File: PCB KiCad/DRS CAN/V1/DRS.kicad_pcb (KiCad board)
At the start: 2 copper layers, 70 x 46.5 mm, 39 parts, among them J1 Screw_Terminal_01x02, J2 Screw_Terminal_01x02, J3 Conn_02x03_Odd_Even, J4 Conn_01x03_Male, J5 Screw_Terminal_01x04, SW1 SW_Push, SW2 SW_Push, SW3 SW_Push, U1 AT90CAN32-16AU, U2 MCP2562-E-SN, U3 LM2596S-5, Y1 Crystal

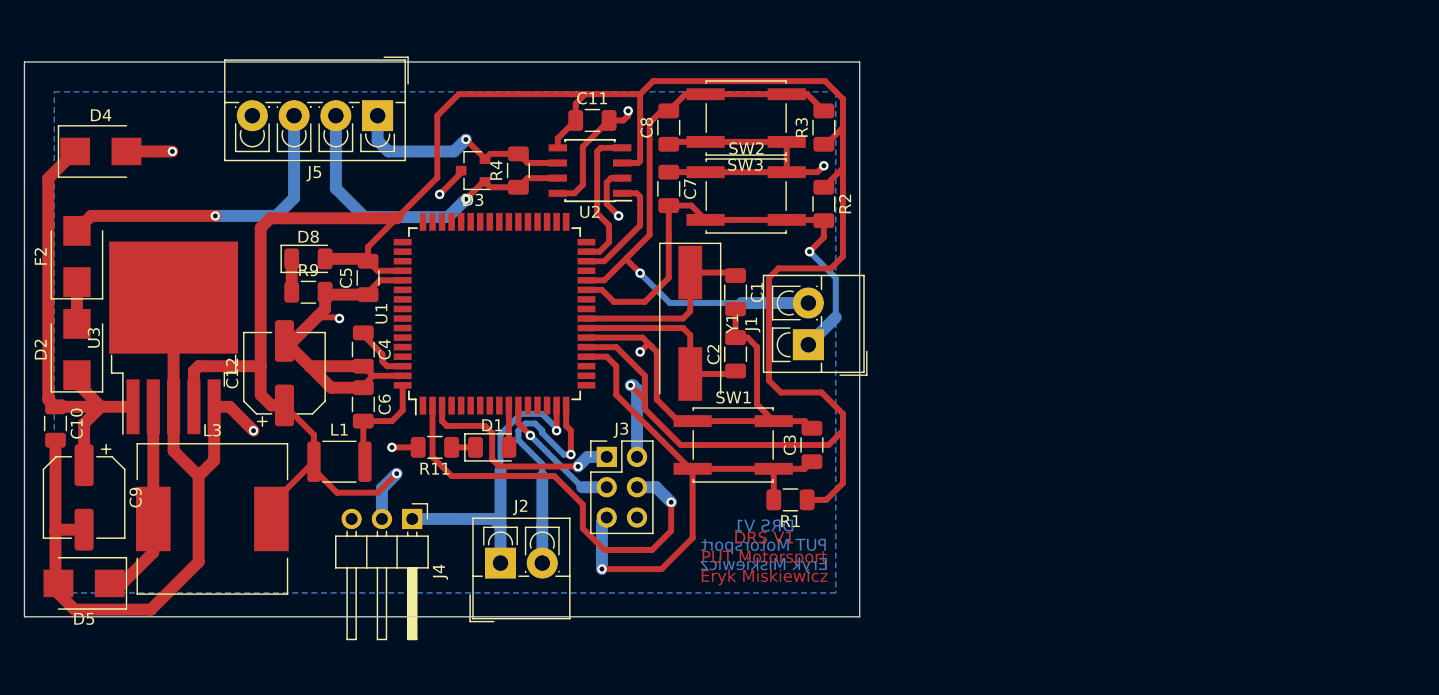
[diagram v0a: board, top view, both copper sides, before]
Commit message: WersjaV2 PCB
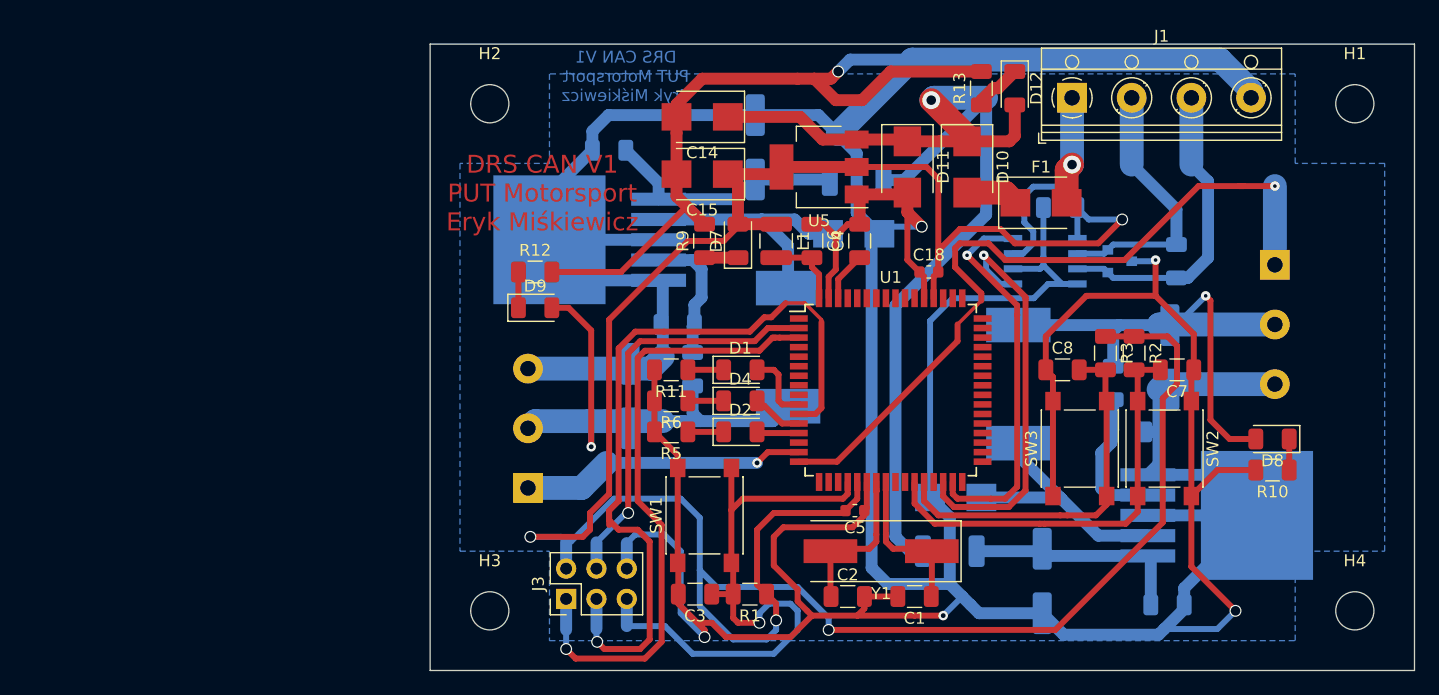
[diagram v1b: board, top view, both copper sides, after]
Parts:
- removed F2: Fuse, Diode_SMD:D_SMB
- removed J5: Screw_Terminal_01x04, TerminalBlock_4Ucon:TerminalBlock_4Ucon_1x04_P3.50mm_Vertical
- added C13: 100n, Capacitor_SMD:C_1206_3216Metric, B.Cu at (109.0, 59.9)
- added C14: CP, Diode_SMD:D_SMB, F.Cu at (116.8, 57.1)
- added C15: CP, Diode_SMD:D_SMB, F.Cu at (116.8, 61.9)
- added C16: 220u, Capacitor_SMD:CP_Elec_6.3x7.7, B.Cu at (156.0, 77.2)
- added C17: 220u, Capacitor_SMD:CP_Elec_6.3x7.7, B.Cu at (110.8, 80.5)
- added C18: 100n, Capacitor_SMD:C_0603_1608Metric, F.Cu at (135.8, 70.1)
- added D10: D_Schottky, Diode_SMD:D_SMB, F.Cu at (139.0, 61.3)
- added D11: D_Zener, Diode_SMD:D_SMB, F.Cu at (134.0, 61.3)
- added D12: LED, LED_SMD:LED_1206_3216Metric, F.Cu at (143.0, 54.7)
- added D6: D_Schottky, Diode_SMD:D_SMB, B.Cu at (129.5, 66.9)
- added D7: LED, LED_SMD:LED_1206_3216Metric, F.Cu at (119.8, 67.5)
- added D9: LED, LED_SMD:LED_1206_3216Metric, F.Cu at (102.8, 73.1)
- added F1: Fuse, Diode_SMD:D_SMB, F.Cu at (145.2, 64.3)
- added H1: MountingHole, MountingHole:MountingHole_3.2mm_M3, F.Cu at (171.5, 56.0)
- added H2: MountingHole, MountingHole:MountingHole_3.2mm_M3, F.Cu at (99.0, 56.0)
- added H3: MountingHole, MountingHole:MountingHole_3.2mm_M3, F.Cu at (99.0, 98.5)
- added H4: MountingHole, MountingHole:MountingHole_3.2mm_M3, F.Cu at (171.5, 98.5)
- added L2: 33u, Inductor_SMD:L_12x12mm_H8mm, B.Cu at (143.3, 79.5)
- added R10: 330, Resistor_SMD:R_1206_3216Metric, F.Cu at (164.6, 86.7)
- added R12: 330, Resistor_SMD:R_1206_3216Metric, F.Cu at (102.8, 70.1)
- added R13: 2k, Resistor_SMD:R_1206_3216Metric, F.Cu at (140.2, 54.7)
- added R14: 0R, Resistor_SMD:R_1206_3216Metric, B.Cu at (152.5, 83.5)
- added R15: 0R, Resistor_SMD:R_1206_3216Metric, B.Cu at (114.8, 74.5)
- added R16: 0R, Resistor_SMD:R_1206_3216Metric, B.Cu at (151.2, 79.4)
- added R17: 0R, Resistor_SMD:R_1206_3216Metric, B.Cu at (116.0, 78.2)
- added R5: 330, Resistor_SMD:R_1206_3216Metric, F.Cu at (114.2, 83.5)
- added R6: 330, Resistor_SMD:R_1206_3216Metric, F.Cu at (114.2, 80.9)
- added R7: 0R, Resistor_SMD:R_2010_5025Metric, B.Cu at (129.8, 62.4)
- added R8: 0R, Resistor_SMD:R_2010_5025Metric, B.Cu at (137.6, 93.5)
- added U4: AP1501-K5G-13, Package_TO_SOT_SMD:TO-263-5_TabPin3, B.Cu at (107.4, 67.4)
- added U5: LM1117-5.0, Package_TO_SOT_SMD:SOT-223-3_TabPin2, F.Cu at (126.6, 61.3)
- C10: value 100n -> 100u; footprint Capacitor_SMD:C_1206_3216Metric -> Capacitor_SMD:CP_Elec_6.3x7.7; moved to B.Cu
- C11, C9, D3, D5, L3, R4, U2: moved to B.Cu
- C12: value 470u/220u -> 100n; footprint Capacitor_SMD:CP_Elec_6.3x7.7 -> Capacitor_SMD:C_1206_3216Metric; moved to B.Cu
- C5: footprint Capacitor_SMD:C_1206_3216Metric -> Capacitor_SMD:C_0603_1608Metric
- D2: value D_Schottky -> LED; footprint Diode_SMD:D_SMB -> LED_SMD:LED_1206_3216Metric
- D4: value D_Zener -> LED; footprint Diode_SMD:D_SMB -> LED_SMD:LED_1206_3216Metric
- J1: value Screw_Terminal_01x02 -> Screw_Terminal_01x04; footprint TerminalBlock_4Ucon:TerminalBlock_4Ucon_1x02_P3.50mm_Vertical -> TerminalBlock_RND:TerminalBlock_RND_205-00014_1x04_P5.00mm_Horizontal
- J2: value Screw_Terminal_01x02 -> Screw_Terminal_01x03; footprint TerminalBlock_4Ucon:TerminalBlock_4Ucon_1x02_P3.50mm_Vertical -> TerminalBlock_RND:TerminalBlock_RND_205-00013_1x03_P5.00mm_Horizontal; moved to B.Cu
- J4: value Conn_01x03_Male -> Screw_Terminal_01x03; footprint Connector_PinHeader_2.54mm:PinHeader_1x03_P2.54mm_Horizontal -> TerminalBlock_RND:TerminalBlock_RND_205-00013_1x03_P5.00mm_Horizontal; moved to B.Cu
- L1: footprint Inductor_SMD:L_1812_4532Metric -> Inductor_SMD:L_1210_3225Metric
- R2, R3: value R -> 10k
- SW1, SW2, SW3: footprint Button_Switch_SMD:SW_SPST_EVQQ2 -> Button_Switch_SMD:SW_SPST_PTS645
- U3: value LM2596S-5 -> AP1501-K5G-13; moved to B.Cu
- moved U3 88.7 mm to (159.9, 90.5), turned to 0 degrees
- moved D8 82.2 mm to (164.6, 84.1), turned to 180 degrees
- moved C9 80.6 mm to (145.3, 96.0)
- moved C12 76.5 mm to (155.8, 98.0), turned to 0 degrees
- moved J4 75.4 mm to (164.8, 69.5)
- moved D5 73.4 mm to (138.1, 89.0)
- moved C10 63.1 mm to (121.2, 59.6), turned to 90 degrees
- moved D4 57.5 mm to (120.0, 80.9)
- moved D2 56.0 mm to (120.0, 83.5), turned to 0 degrees
- moved R4 55.7 mm to (156.6, 69.2)
- moved D3 54.7 mm to (151.8, 69.2), turned to 0 degrees
- moved L3 50.4 mm to (124.0, 76.4), turned to 270 degrees
- moved C5 45.2 mm to (129.6, 90.1), turned to 180 degrees
- moved C7 45.2 mm to (156.6, 78.3), turned to 180 degrees
- moved C4 42.6 mm to (130.0, 67.5), turned to 90 degrees
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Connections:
- net /LED renamed /LED1
- C10 pad 1: +12P -> /Zasilanie/12L
- C12 pad 1: +5V -> /Zasilanie/12P
- C9 pad 1: +12P -> /Zasilanie/12P
- D2 pad 1: +12P -> Net-(D2-Pad1)
- D2 pad 2: Net-(D2-Pad2) -> /LED3
- D4 pad 1: +12P -> Net-(D4-Pad1)
- D4 pad 2: GND -> /LED2
- D5 pad 1: Net-(D5-Pad1) -> /Zasilanie/5PU
- D8 pad 2: +5V -> +5VP
- J1 pad 1: /Button1 -> +12P
- J1 pad 2: /Button2 -> /CANL
- J2 pad 2: /PWM2 -> +5VL
- J4 pad 1: /PWM1 -> /PWM2
- J4 pad 2: +5V -> +5VP
- L3 pad 1: Net-(D5-Pad1) -> /Zasilanie/5LU
- L3 pad 2: +5V -> +5VL
- R9 pad 1: Net-(D8-Pad1) -> Net-(D7-Pad1)
- U1 pad 12: (no net) -> /LED2
- U1 pad 13: (no net) -> /LED3
- U3 pad 1: +12P -> /Zasilanie/12P
- U3 pad 2: Net-(D5-Pad1) -> /Zasilanie/5PU
- U3 pad 4: +5V -> Net-(R14-Pad2)
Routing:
- net GND: track 183.2 -> 527.5 mm, vias 9 -> 6
- net +12V: track 26.3 -> 91.3 mm
- net /SCK: track 11.1 -> 65.1 mm
- net +5VP: track 0.00 -> 43.6 mm, vias 0 -> 1
- net /PWM2: track 22.0 -> 64.1 mm
- net +5VL: track 0.00 -> 41.8 mm, vias 0 -> 1
- net /MISO: track 18.3 -> 52.1 mm
- net +12P: track 38.0 -> 8.99 mm, vias 0 -> 1
- net /TXCAN: track 9.76 -> 34.2 mm, vias 0 -> 1
- net /Zasilanie/5PU: track 0.00 -> 21.5 mm
- net /Zasilanie/5LU: track 0.00 -> 21.4 mm
- net /Zasilanie/12L: track 0.00 -> 20.3 mm
- net /RXCAN: track 12.5 -> 32.6 mm, vias 0 -> 1
- net /Zasilanie/12P: track 0.00 -> 18.9 mm
- net /Button2: track 49.3 -> 31.3 mm, vias 1 -> 0
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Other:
- board size 70 x 46.5 mm -> 82.5 x 52.5 mm
- board text added: "DRS CAN V1 PUT Motorsport Eryk Miśkiewicz"
- board text removed: "DRS V1 PUT Motorsport Eryk Miskiewicz"
